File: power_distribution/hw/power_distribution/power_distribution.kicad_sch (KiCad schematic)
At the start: 8 parts, among them J1 Conn_01x02, Q1 P-MOSFET 60V

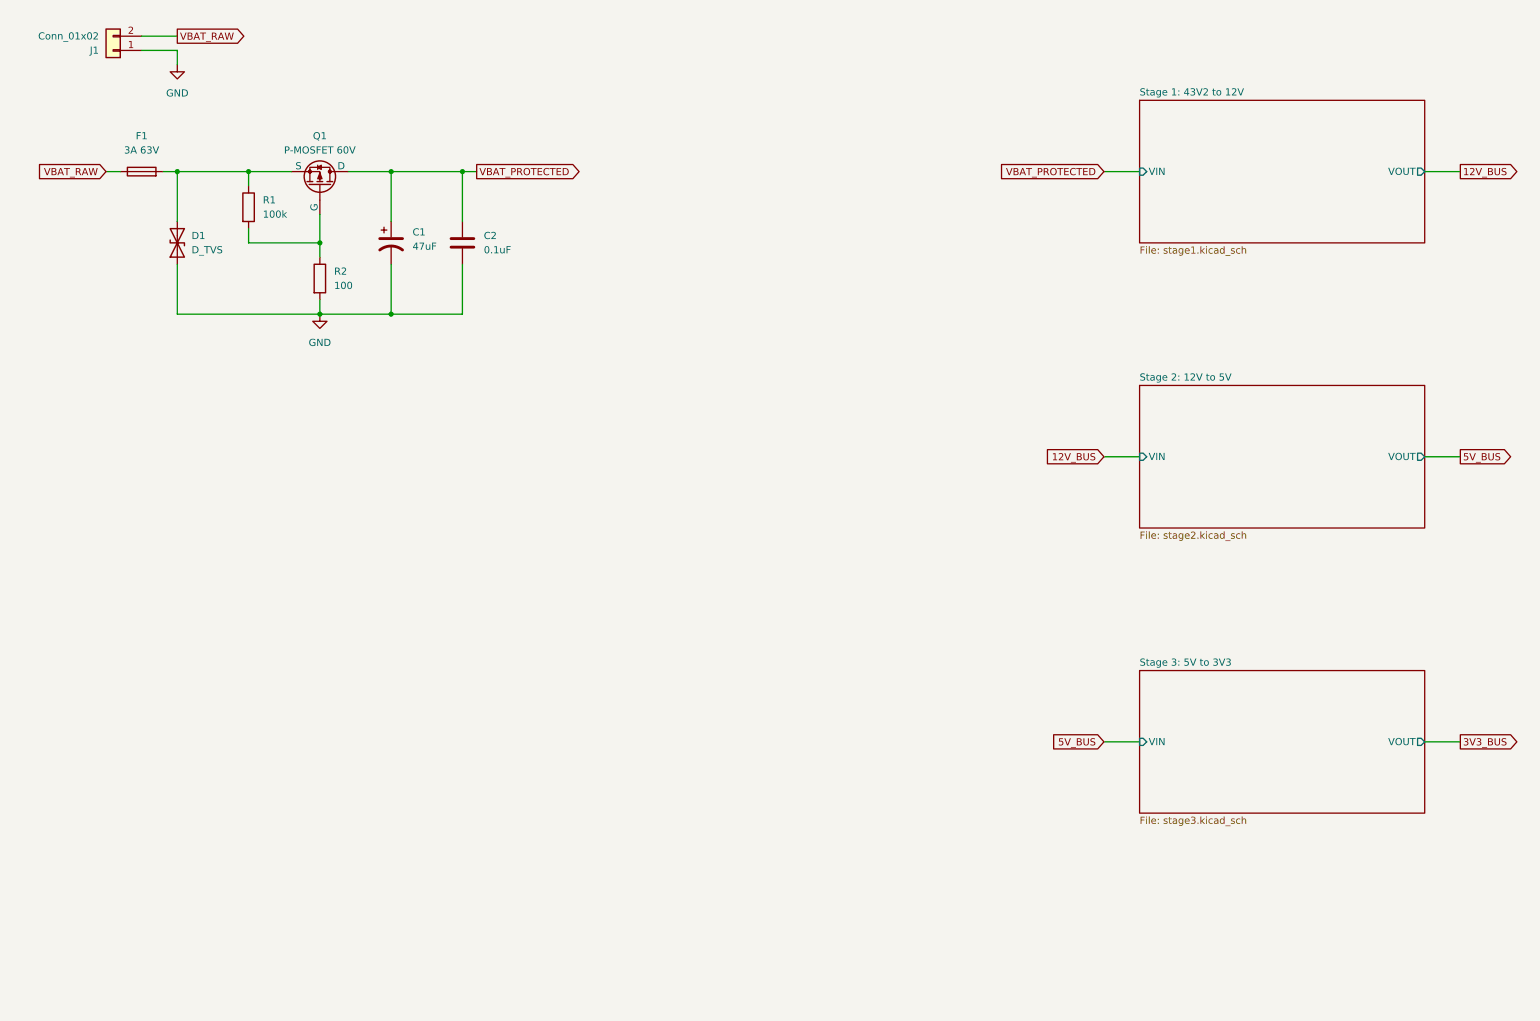
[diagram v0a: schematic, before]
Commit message: Finish Input stage
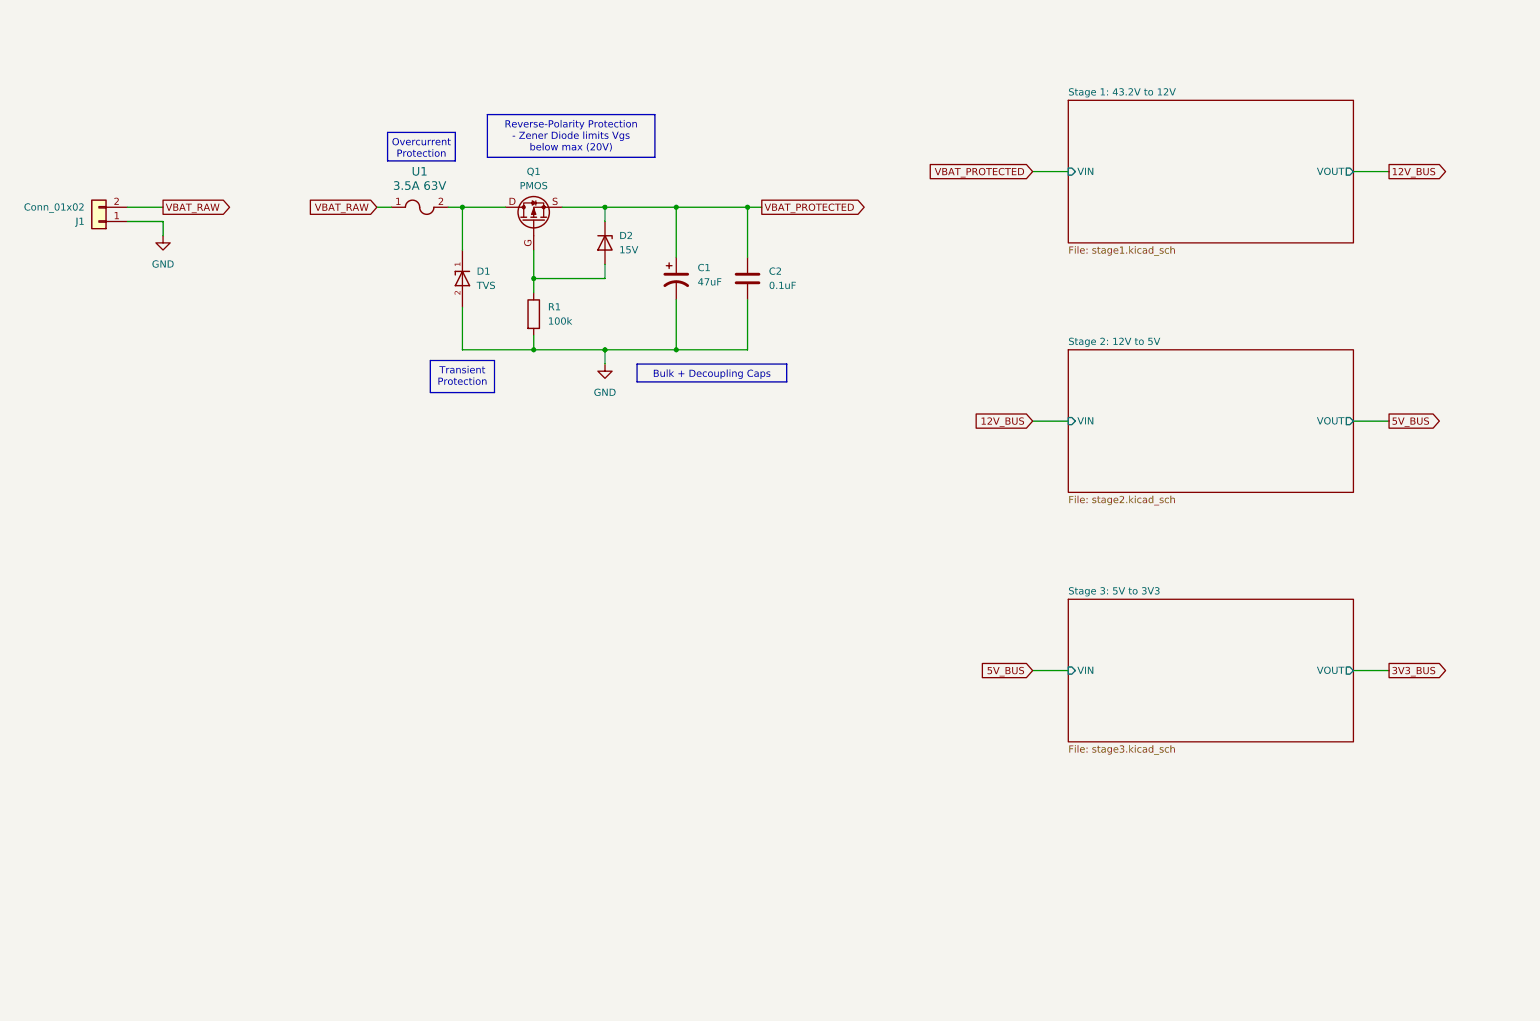
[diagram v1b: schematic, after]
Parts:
- removed D1: D_TVS, symbol Device:D_TVS
- removed F1: 3A 63V, symbol Device:Fuse
- removed R2: 100, symbol Device:R
- added D1: TVS, SMBJ51A-13-F:DIOM5336X250N, symbol SMBJ51A-13-F:SMBJ51A-13-F
- added D2: 15V, BZT52C15-7-F:SOD3715X135N, symbol Device:D_Zener
- added U1: 3.5A 63V, C1_BEL, symbol 0685T3500-01:C1T_3.5
- Q1: value P-MOSFET 60V -> PMOS; footprint (none) -> GSFD6959:PMOSGDS_TO-252_DPAK_GAS
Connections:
- net GND: now also R1.2, D1.2
- net VBAT_PROTECTED: now also Q1.S, D2.1 (K); no longer Q1.D
- net VBAT_RAW: now also U1.1
- net at R1.1: now also Q1.G, D2.2 (A); no longer Q1.S
- new net: D1.1, Q1.D, U1.2
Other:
- sheet Stage 1: 43V2 to 12V renamed Stage 1: 43.2V to 12V
- moved on the sheet: C1, C2, J1, R1

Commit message: Finish output stage
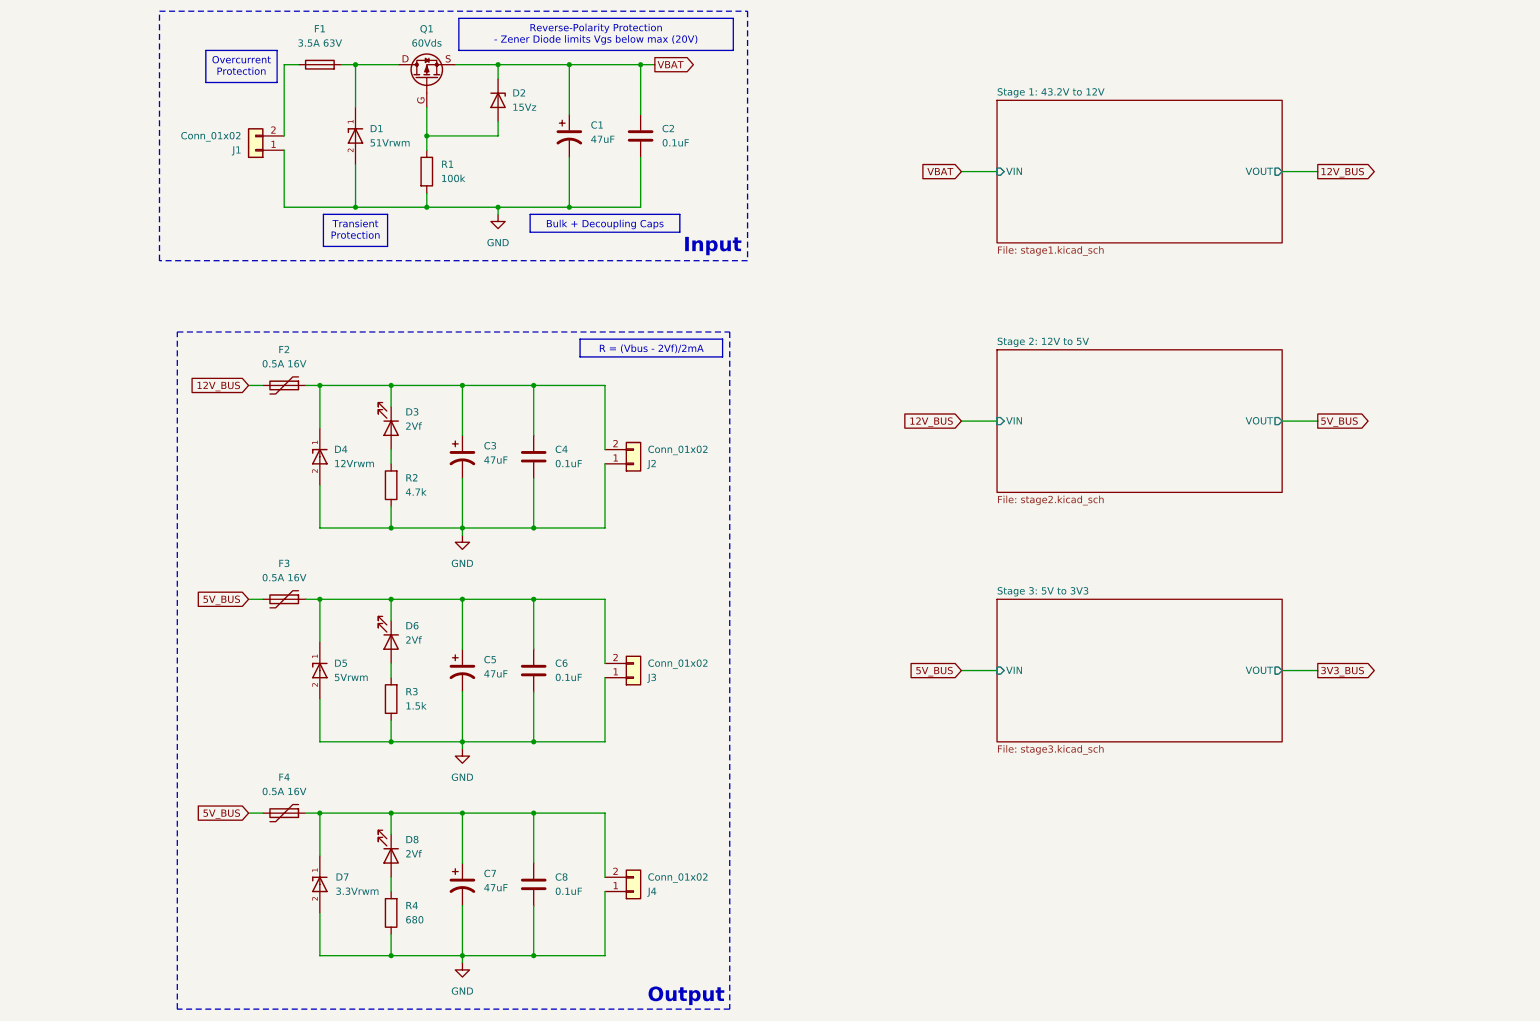
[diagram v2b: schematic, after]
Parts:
- removed U1: 3.5A 63V, C1_BEL, symbol 0685T3500-01:C1T_3.5
- added C3, C5, C7: 47uF, symbol Device:C_Polarized_US
- added C4, C6, C8: 0.1uF, symbol Device:C
- added D3, D6, D8: 2Vf, symbol Device:LED
- added D4: 12Vrwm, ESD5Z12T1G:SOD-523_0P9X1P3_ONS, symbol SMBJ51A-13-F:SMBJ51A-13-F
- added D5: 5Vrwm, ESD5Z5.0T1G:SOD-523_0P9X1P3_ONS, symbol SMBJ51A-13-F:SMBJ51A-13-F
- added D7: 3.3Vrwm, ESD5Z5.0T1G:SOD-523_0P9X1P3_ONS, symbol SMBJ51A-13-F:SMBJ51A-13-F
- added F1: 3.5A 63V, 0685T3500-01:C1_BEL, symbol Device:Fuse
- added F2, F3, F4: 0.5A 16V, 0ZCH0050FF2G:0ZCH_BEL, symbol Device:Polyfuse
- added J2, J3, J4: Conn_01x02, Connector_JST:JST_PH_S2B-PH-K_1x02_P2.00mm_Horizontal, symbol Connector_Generic:Conn_01x02
- added R2: 4.7k, symbol Device:R
- added R3: 1.5k, symbol Device:R
- added R4: 680, symbol Device:R
- D1: value TVS -> 51Vrwm
- D2: value 15V -> 15Vz
- Q1: value PMOS -> 60Vds
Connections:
- net 12V_BUS: now also F2.2
- net 5V_BUS: now also F3.2, F4.2
- net GND: now also C3.2, C4.2, C5.2, C6.2, C7.2, C8.2, D4.2, D5.2, D7.2, J2.1 (Pin_1), J3.1 (Pin_1), J4.1 (Pin_1), R2.1, R3.1, R4.1
- net at D1.1, Q1.D: now also F1.2
- net VBAT_PROTECTED renamed VBAT
- net VBAT_RAW: no longer names the net of J1.2 (Pin_2)
- net VBAT_RAW: now also F1.1
- new net: C3.1, C4.1, D3.1 (K), D4.1, F2.1, J2.2 (Pin_2)
- new net: C7.1, C8.1, D7.1, D8.1 (K), F4.1, J4.2 (Pin_2)
- new net: C5.1, C6.1, D5.1, D6.1 (K), F3.1, J3.2 (Pin_2)
- new net: D3.2 (A), R2.2
- new net: D6.2 (A), R3.2
- new net: D8.2 (A), R4.2
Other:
- note added: "Input"
- note added: "Output"
- moved on the sheet: C1, C2, D1, D2, J1, Q1, R1
